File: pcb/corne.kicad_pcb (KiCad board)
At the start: 2 copper layers, 134.3 x 93.5 mm, 105 parts, among them J1 TYPE-C-31-M-13C, J2 ST-0277D00-052-142, J3 Conn_01x04, J4 Conn_01x03, SW1 SW_Push, SW10 SW_Push, SW11 SW_Push, SW12 SW_Push, SW13 SW_Push, SW14 SW_Push, SW15 SW_Push, SW16 SW_Push, SW17 SW_Push, SW18 SW_Push, SW19 SW_Push, SW2 SW_Push, SW20 SW_Push, SW21 SW_Push, SW3 SW_Push, SW4 SW_Push, SW5 SW_Push, SW6 SW_Push, SW7 SW_Push, SW8 SW_Push, SW9 SW_Push, U1 RP2040, U2 NCP1117LPST33T3G, U3 TPD4E05U06DQAR, U4 W25Q128JVSIQ, Y1 12MHz 10pF

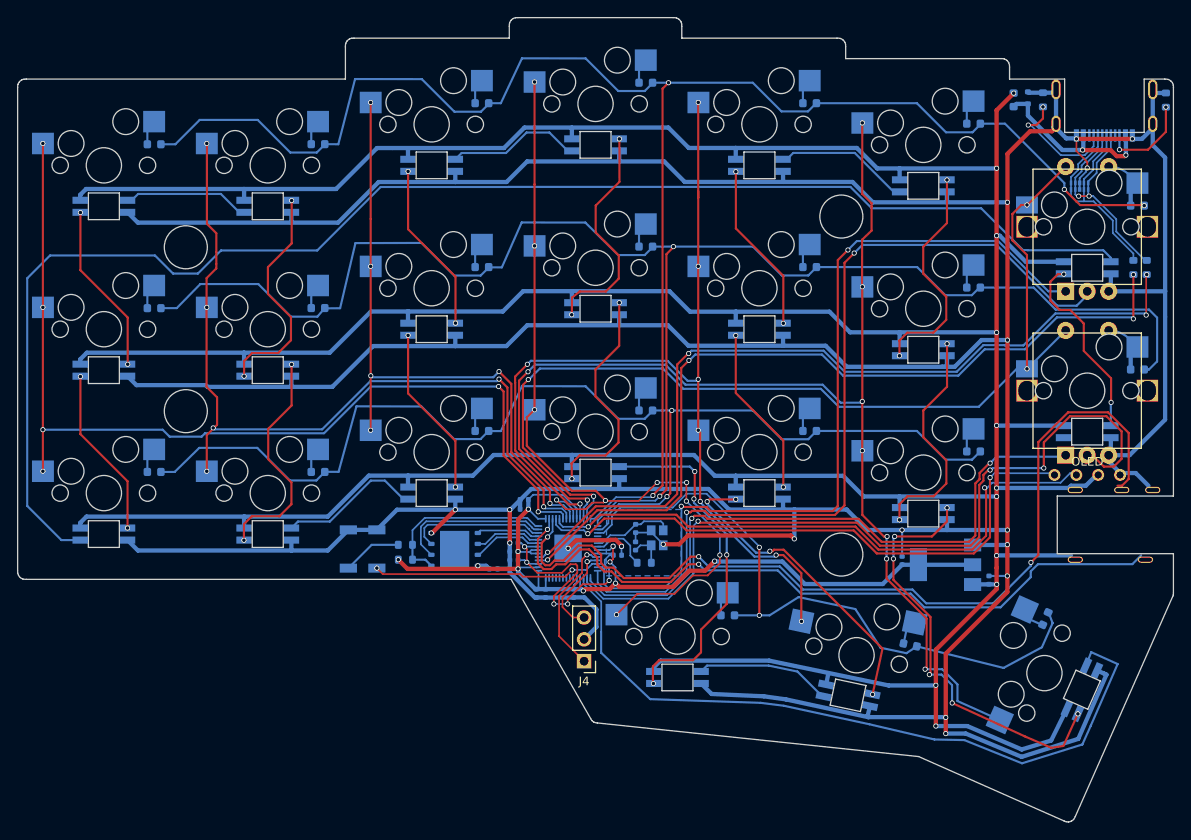
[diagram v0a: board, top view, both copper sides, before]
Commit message: Update lines
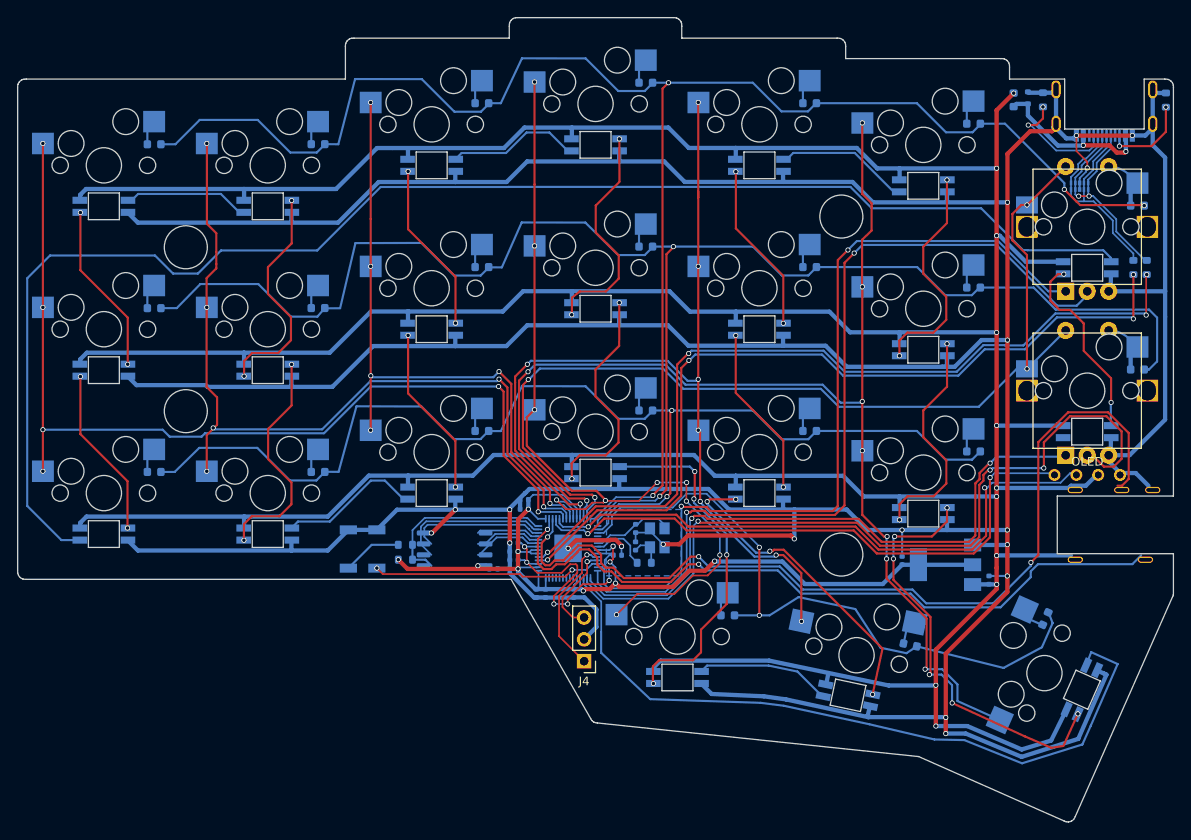
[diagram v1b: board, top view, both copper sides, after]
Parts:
- C1, C2: value 20p -> 27p
- U4: footprint Package_SON:WSON-8-1EP_6x5mm_P1.27mm_EP3.4x4.3mm -> Package_SO:SOIC-8_5.23x5.23mm_P1.27mm
- Y1: value 12MHz 10pF -> 12MHz 18pF; footprint Crystal:Crystal_SMD_2520-4Pin_2.5x2.0mm -> Crystal:Crystal_SMD_3225-4Pin_3.2x2.5mm
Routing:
- net VBUS: track 19.8 -> 18.6 mm
- net Net-(J1-CC2): track 10.4 -> 9.79 mm
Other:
- outline, holes or cut-outs redrawn
